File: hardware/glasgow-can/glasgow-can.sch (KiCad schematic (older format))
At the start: 6 parts, among them J1 Conn_02x10_Odd_Even, J2 A-DS 09 A/KG-T2S, J3 Conn_01x09_Male, J4 Conn_01x03_Male, J5 Conn_02x10_Odd_Even, J6 Conn_01x03

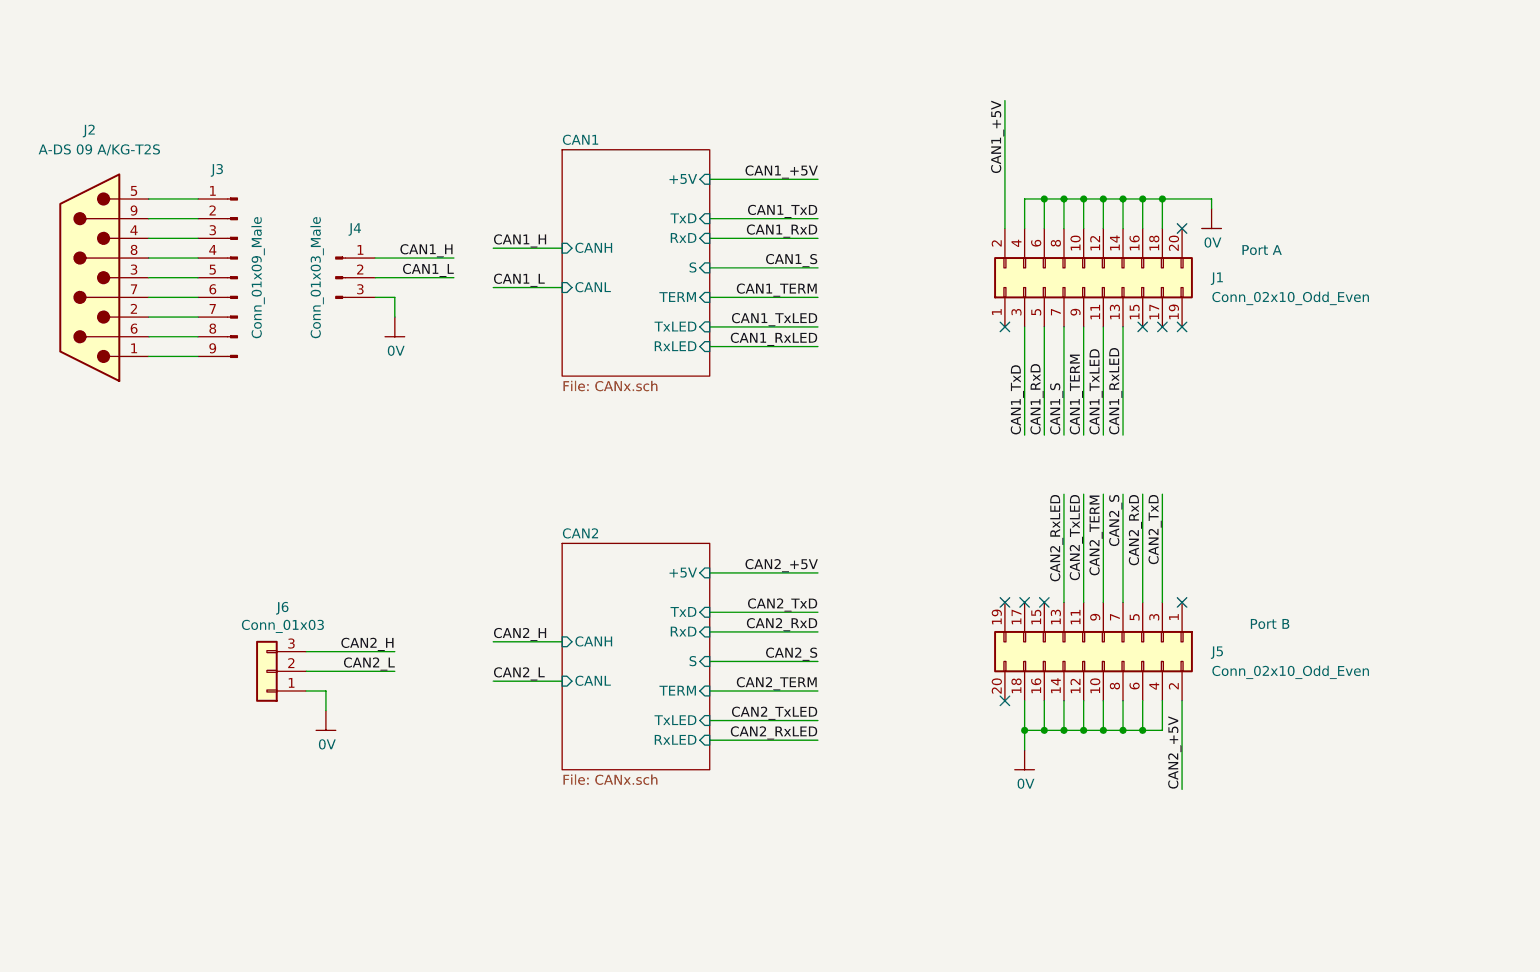
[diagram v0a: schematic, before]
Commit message: tidy up schematics
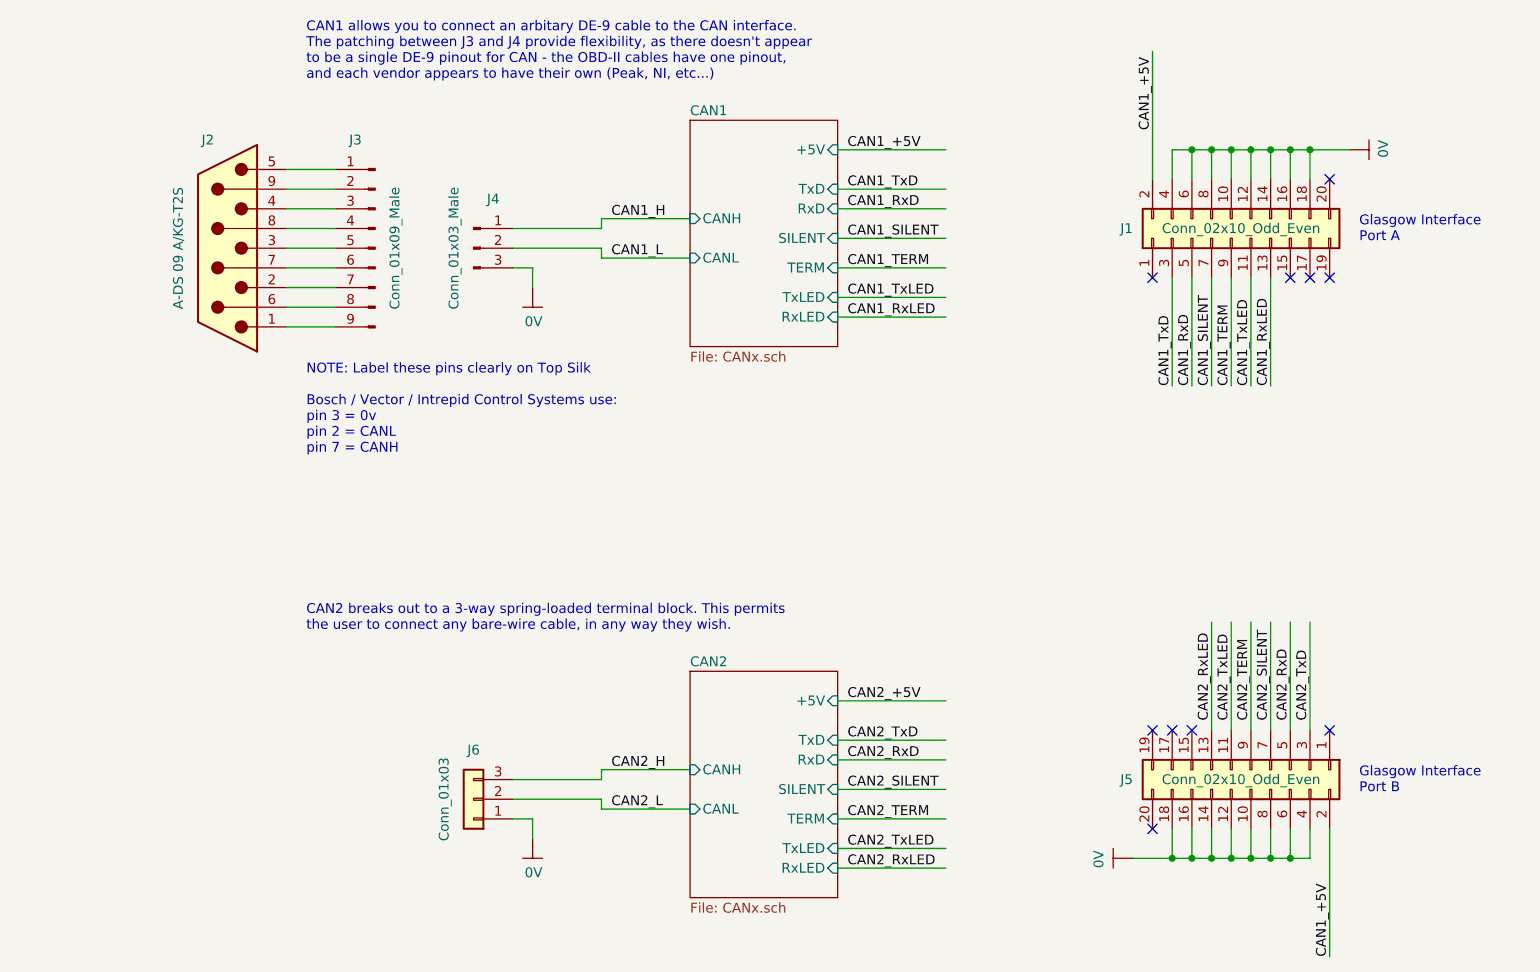
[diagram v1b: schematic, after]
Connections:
- net labels added: CAN1_SILENT, CAN2_SILENT
- net labels removed: CAN1_S, CAN2_S
- wire segments 82 -> 85
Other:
- note added: "CAN1 allows you to connect an arbitary DE-9 cable to the CAN interface.\nThe patching between J3 and J4 provide flexibility, as there doesn't appear\nto be a single DE-9 pinout for CAN - the OBD-II cables have one pinout,\nand each vendor appears to have their own (Peak, NI, etc...)"
- note added: "CAN2 breaks out to a 3-way spring-loaded terminal block. This permits\nthe user to connect any bare-wire cable, in any way they wish."
- note added: "Glasgow Interface\nPort A"
- note added: "Glasgow Interface\nPort B"
- note added: "NOTE: Label these pins clearly on Top Silk\n\nBosch / Vector / Intrepid Control Systems use:\npin 3 = 0v\npin 2 = CANL\npin 7 = CANH"
- note removed: "Port A"
- note removed: "Port B"
- moved on the sheet: J1, J2, J3, J4, J5, J6
